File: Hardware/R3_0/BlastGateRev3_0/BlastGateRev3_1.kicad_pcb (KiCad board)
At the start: 2 copper layers, 51.9 x 54.5 mm, 45 parts, among them J1 Conn_01x03_Male, J2 Conn_01x06_Male, J3 USB_B_Micro, J4 RJ9, J5 Conn_01x03_Male, SW1 SW_DIP_x03, SW2 SW_SPDT_MSM, SW4 SW_SPDT_MSM, U1 AP2112M-3.3, U2 ESP32-WROOM-32D

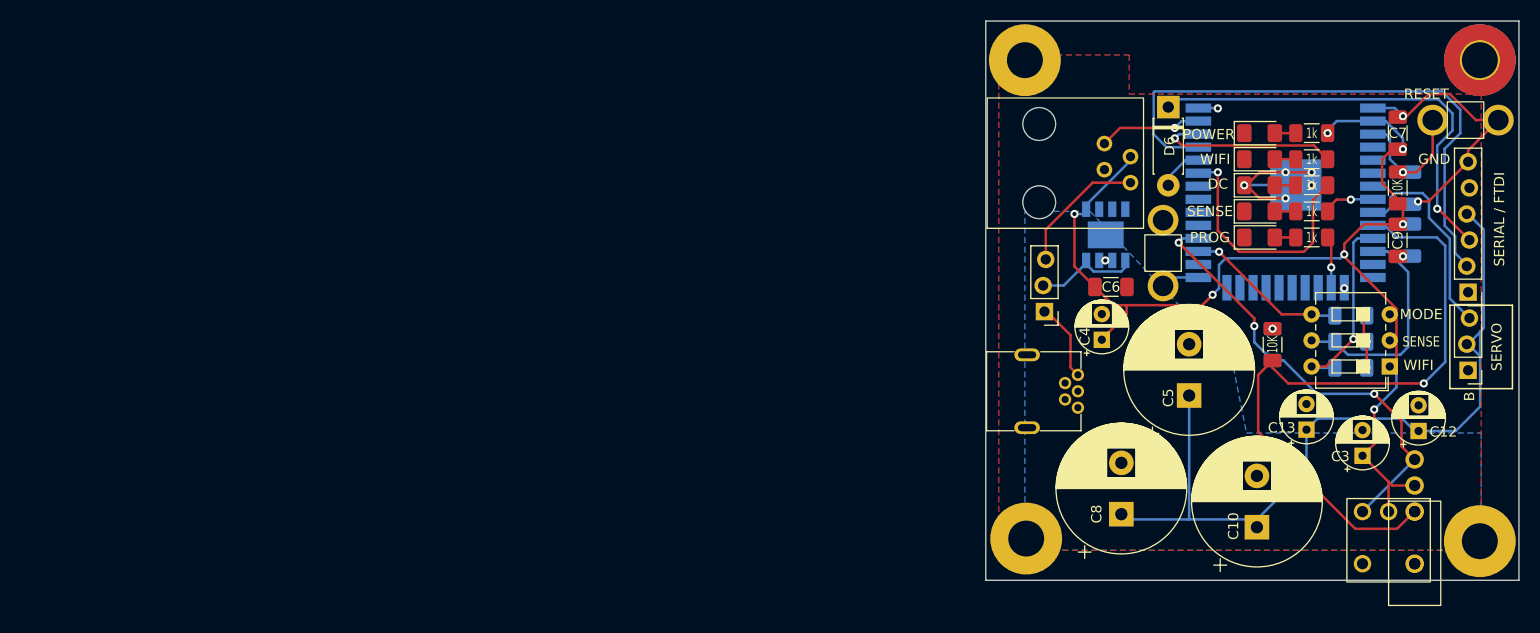
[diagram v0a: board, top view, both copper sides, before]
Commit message: hardware revision,
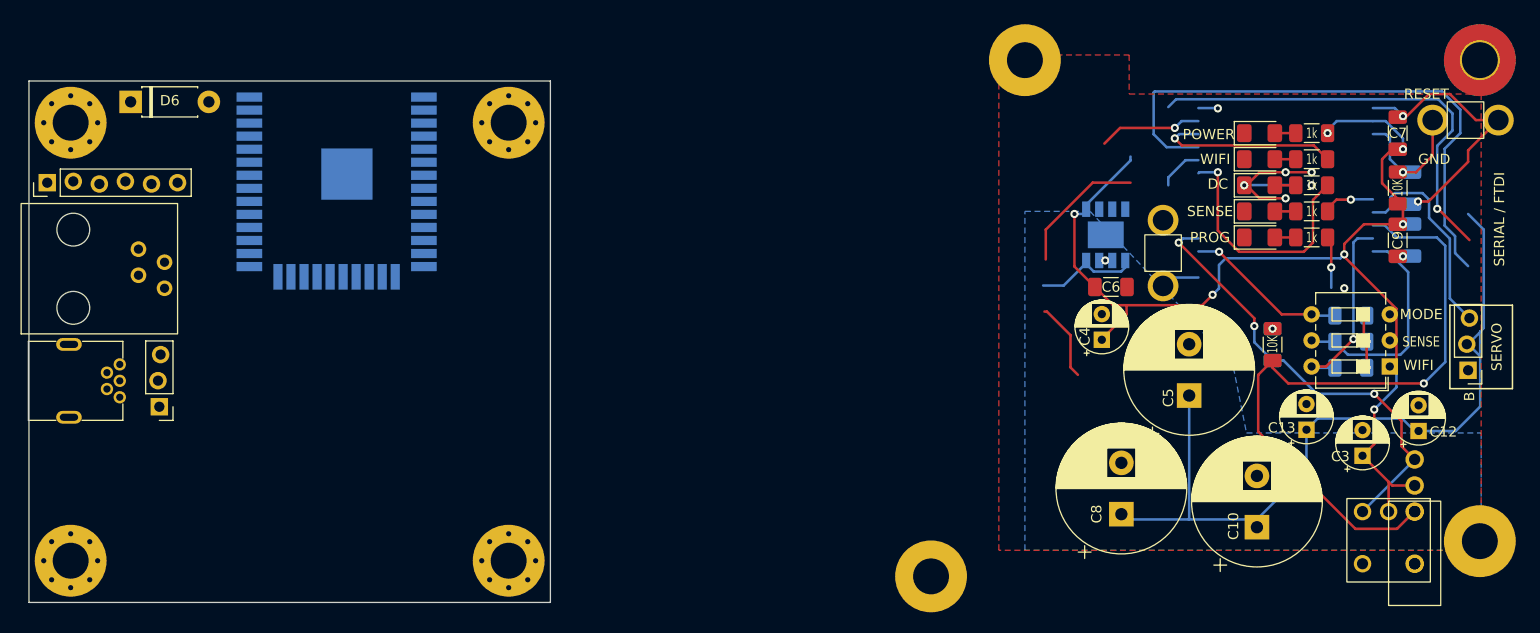
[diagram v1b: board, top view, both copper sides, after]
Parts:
- added REF**: MountingHole_3.5mm_Pad_Via, MountingHole:MountingHole_3.5mm_Pad_Via, F.Cu at (122.4, 107.7)
- added REF**: MountingHole_3.5mm_Pad_Via, MountingHole:MountingHole_3.5mm_Pad_Via, F.Cu at (122.4, 65.0)
- added REF**: MountingHole_3.5mm_Pad_Via, MountingHole:MountingHole_3.5mm_Pad_Via, F.Cu at (79.8, 65.0)
- added REF**: MountingHole_3.5mm_Pad_Via, MountingHole:MountingHole_3.5mm_Pad_Via, F.Cu at (79.8, 107.7)
- moved J2 138.8 mm to (77.5, 70.9), turned to 90 degrees
- moved D6 101.1 mm to (85.6, 63.0), turned to 0 degrees
- moved J4 94.7 mm to (80.0, 75.4)
- moved J3 93.4 mm to (75.6, 90.2)
- moved U2 92.5 mm to (105.7, 70.8)
- moved J5 86.7 mm to (88.4, 92.7)
- moved REF** 9.98 mm to (163.6, 109.2)
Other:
- board size 51.9 x 54.5 mm -> 50.8 x 50.8 mm
